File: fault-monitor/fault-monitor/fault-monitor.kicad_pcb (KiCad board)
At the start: 2 copper layers, 72 x 73.5 mm, 25 parts, among them J1 Conn_01x03, J2 Conn_01x06, J3 Conn_01x02, J4 Conn_01x02, J5 Conn_01x02, J6 Conn_01x02, J7 Conn_01x06, U1 ESP32-DevKitC

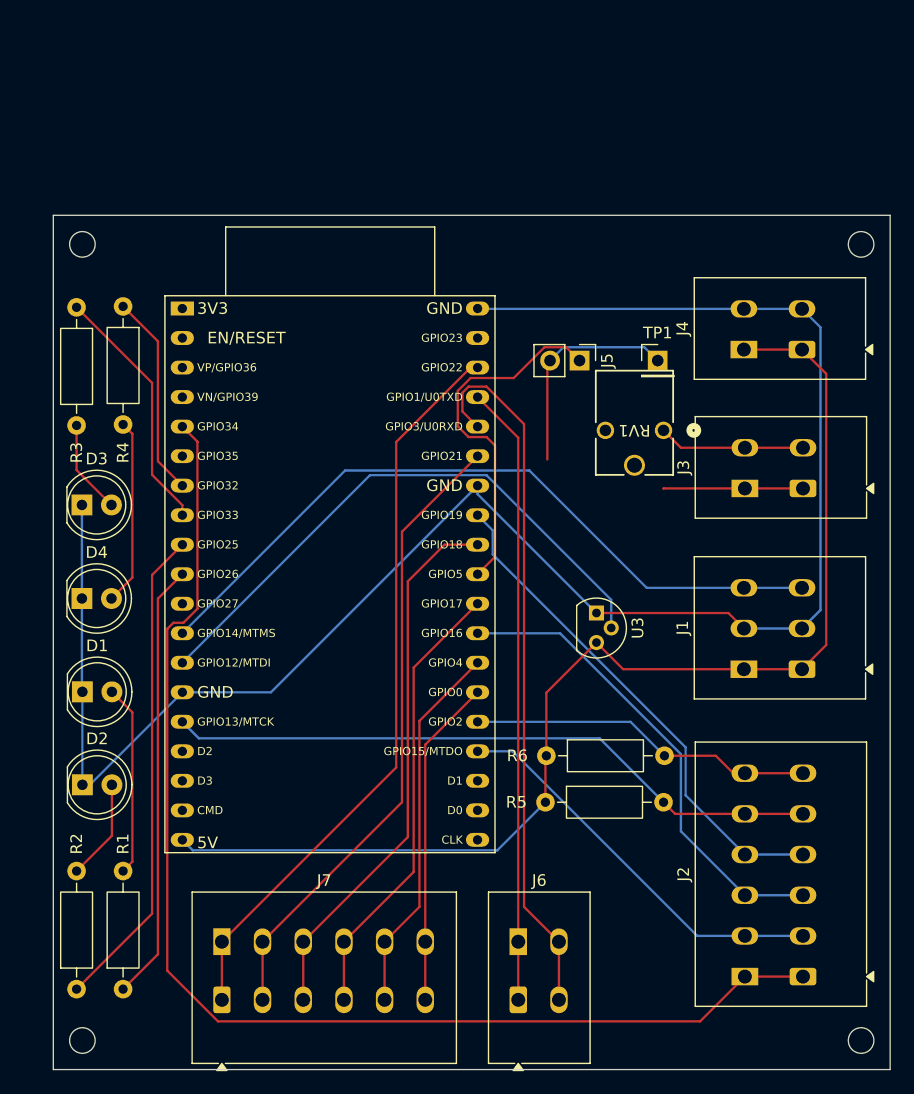
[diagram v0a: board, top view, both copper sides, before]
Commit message: full redo of pcb cuz we fucked up the usb port
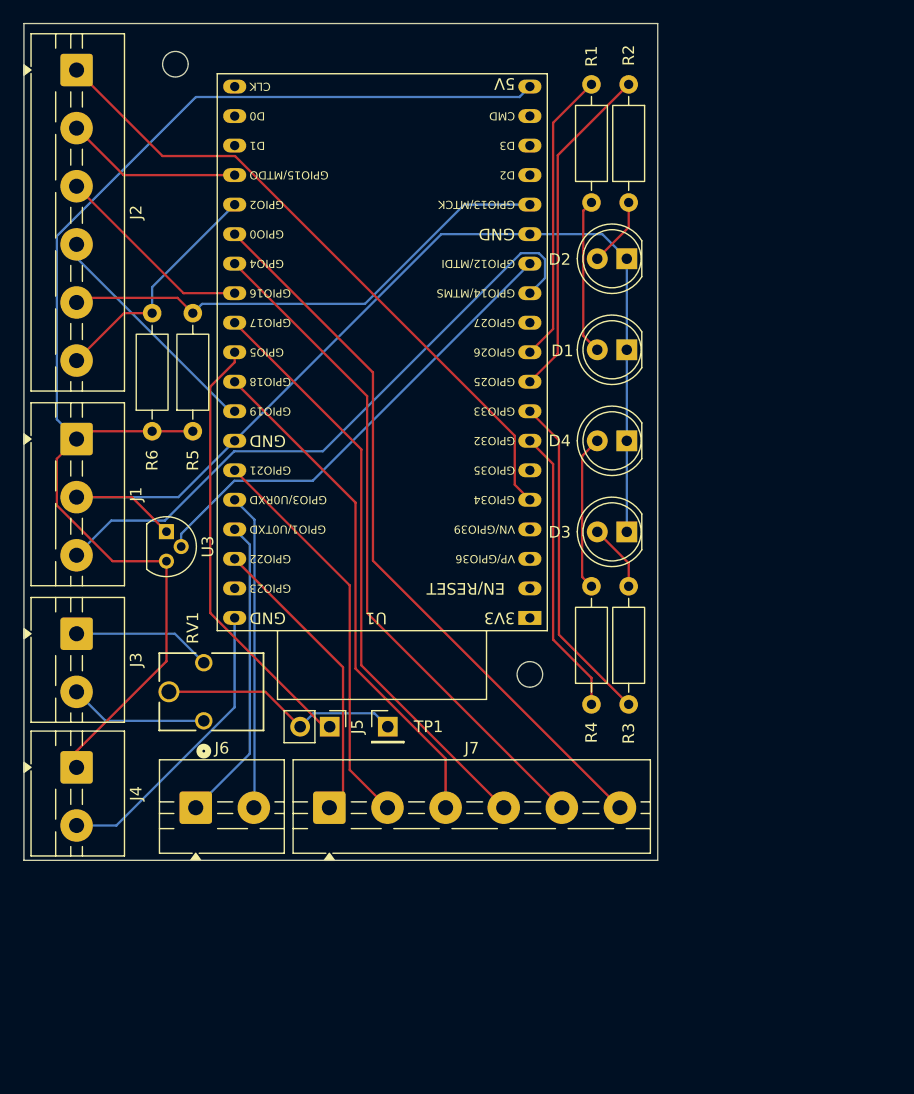
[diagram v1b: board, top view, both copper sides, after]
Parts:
- removed the REF** at (120.5, 43.0)
- removed the REF** at (53.5, 111.5)
- removed the REF** at (53.5, 43.0)
- removed the REF** at (120.5, 111.5)
- added REF**: MountingHole_2.2mm_M2, MountingHole:MountingHole_2.2mm_M2, F.Cu at (61.5, 27.5)
- added REF**: MountingHole_2.2mm_M2, MountingHole:MountingHole_2.2mm_M2, F.Cu at (92.0, 80.0)
- J1: footprint TerminalBlock_WAGO_3D:TerminalBlock_WAGO_2601-1103_1x03_P3.50mm_Horizontal-3D -> TerminalBlock:TerminalBlock_MaiXu_MX126-5.0-03P_1x03_P5.00mm
- J2, J7: footprint TerminalBlock_WAGO_3D:TerminalBlock_WAGO_2601-1106_1x06_P3.50mm_Horizontal-3D -> TerminalBlock:TerminalBlock_MaiXu_MX126-5.0-06P_1x06_P5.00mm
- J3, J4, J6: footprint TerminalBlock_WAGO_3D:TerminalBlock_WAGO_2601-1102_1x02_P3.50mm_Horizontal-3D -> TerminalBlock:TerminalBlock_MaiXu_MX126-5.0-02P_1x02_P5.00mm
- moved J2 100.0 mm to (53.0, 28.0), turned to -90 degrees
- moved R2 91.2 mm to (100.5, 29.2), turned to -90 degrees
- moved R1 87.7 mm to (97.3, 29.2), turned to -90 degrees
- moved J4 72.0 mm to (53.0, 88.0), turned to -90 degrees
- moved J1 65.5 mm to (53.0, 59.8), turned to -90 degrees
- moved D2 65.1 mm to (100.3, 44.2), turned to 180 degrees
- moved J3 63.7 mm to (53.0, 76.5), turned to -90 degrees
- moved R3 58.5 mm to (100.5, 82.6), turned to 90 degrees
- moved D1 55.3 mm to (100.3, 52.1), turned to 180 degrees
- moved R4 52.9 mm to (97.3, 82.6), turned to 90 degrees
- moved D4 48.8 mm to (100.3, 59.9), turned to 180 degrees
- moved D3 46.9 mm to (100.3, 67.7), turned to 180 degrees
- moved RV1 46.8 mm to (63.9, 84.0), turned to 90 degrees
- moved R5 44.0 mm to (63.0, 59.1), turned to 90 degrees
- moved R6 43.9 mm to (59.5, 59.1), turned to 90 degrees
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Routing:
- net /STOPALL: track 107.0 -> 56.8 mm
- net GND: track 158.9 -> 115.6 mm
- net /IO22: track 63.9 -> 25.8 mm
- net /IO0: track 28.3 -> 63.1 mm
- net Net-(J6-Pin_2): track 61.1 -> 27.2 mm
- net Net-(J6-Pin_1): track 53.3 -> 26.4 mm
- net /IO4: track 32.3 -> 58.5 mm
- net /SOFTSTART: track 41.2 -> 17.4 mm
- net /FAN: track 43.7 -> 20.2 mm
- net /IO21: track 54.4 -> 34.5 mm
- net /RELAY: track 34.6 -> 15.3 mm
- net /ALARMLEFT: track 56.7 -> 43.6 mm
- net Net-(U1-IO25): track 42.0 -> 29.1 mm
- net Net-(U1-IO26): track 37.8 -> 25.2 mm
- net /IO17: track 38.8 -> 51.3 mm
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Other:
- board size 72 x 73.5 mm -> 54.5 x 72 mm
- board text removed: "0"
- board text removed: "17"
- board text removed: "18"
- board text removed: "21"
- board text removed: "22"
- board text removed: "24V"
- board text removed: "24V REF"
- board text removed: "4"
- board text removed: "5V"
- board text removed: "5V PWR"
- board text removed: "ALL"
- board text removed: "ALR"
- board text removed: "CURR. SENS."
- board text removed: "FAN"
- board text removed: "GND"
- board text removed: "GPIO"
- board text removed: "IN"
- board text removed: "REL"
- board text removed: "RX"
- board text removed: "SNS"
- board text removed: "SST"
- board text removed: "STP"
- board text removed: "TX"
